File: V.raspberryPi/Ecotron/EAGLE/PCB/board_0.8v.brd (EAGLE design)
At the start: 65.8 x 31.6 mm, 35 parts, among them J1 1X2-3.5MM, J2 1X2-3.5MM, J3 1X2-3.5MM, J4 4P-2.0, J5 4P-2.0, J6 4P-2.0, J7 4P-2.0, T1 T1, T2 T2, T4 MOSFET-N, T6 MOSFET-N, U1 ADS1015, U2 PCA9685, U3 TXB0108, U4 PCA9546APW,112

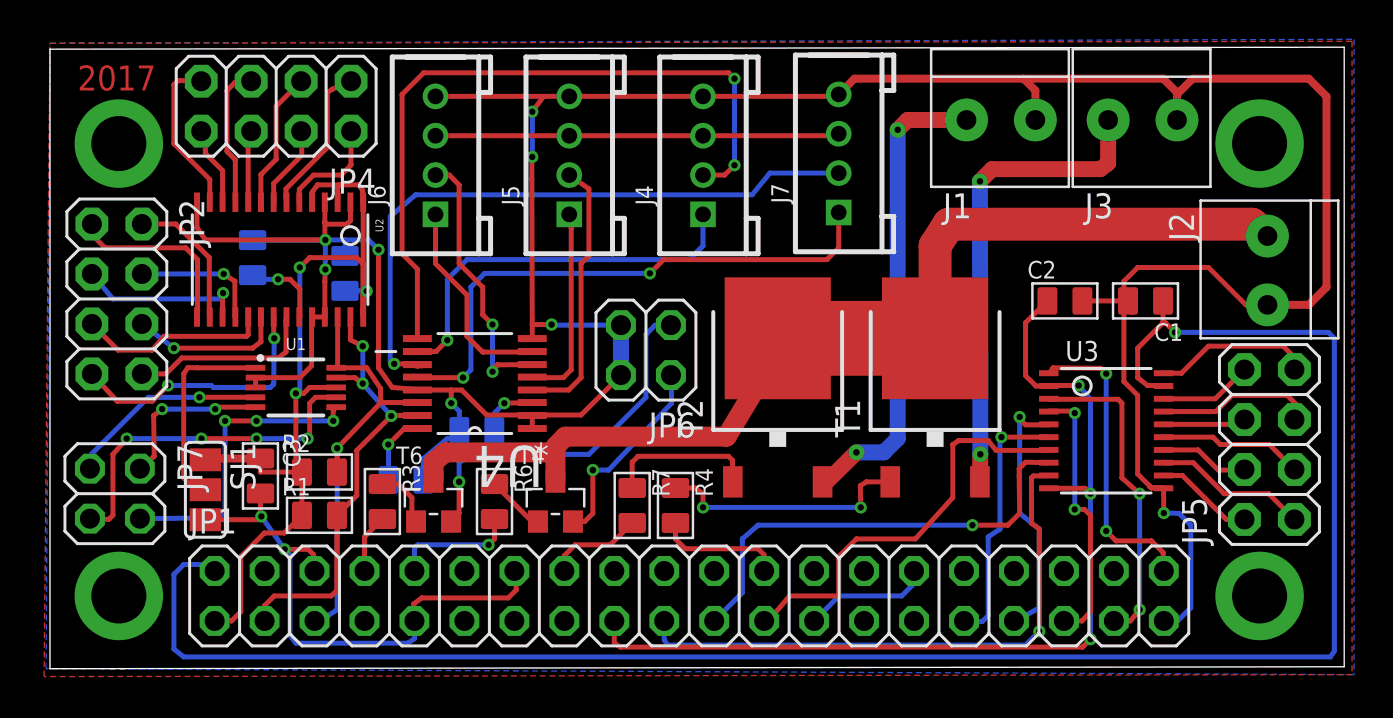
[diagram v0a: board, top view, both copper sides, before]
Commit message: update board
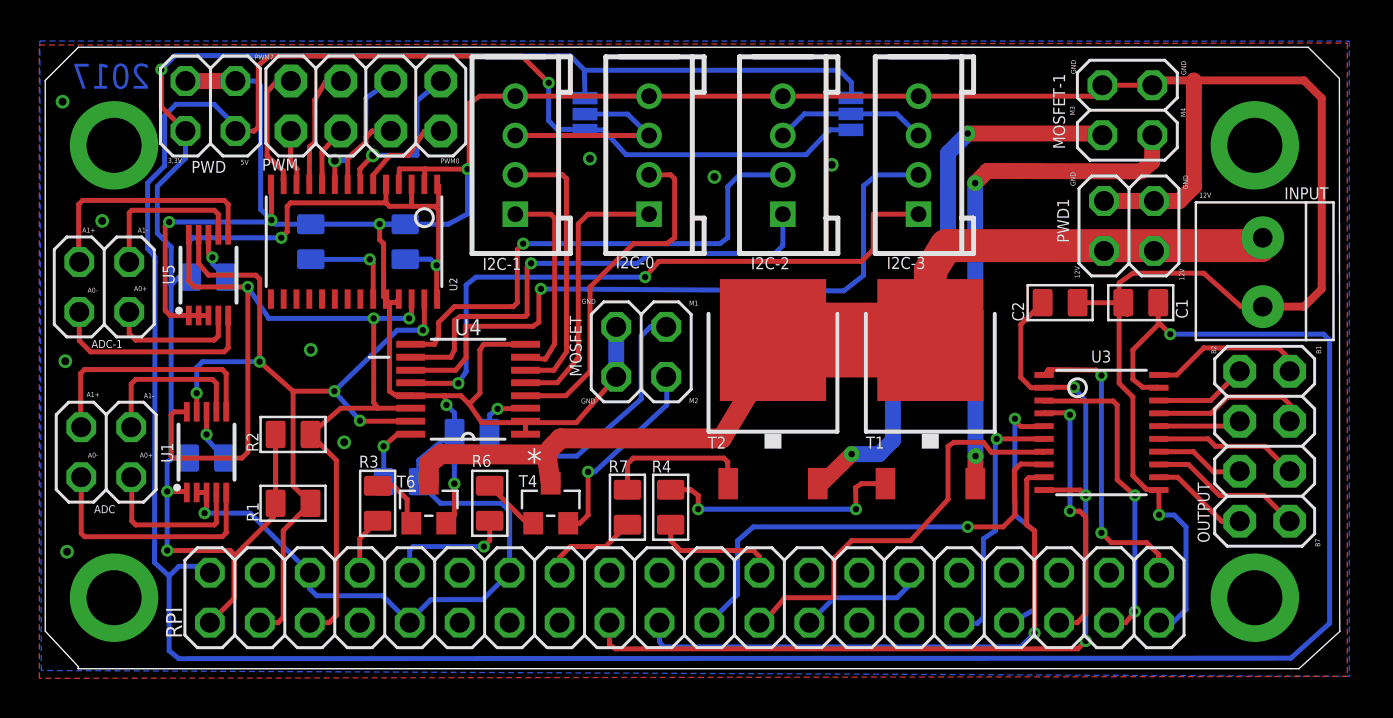
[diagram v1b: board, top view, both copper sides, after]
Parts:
- removed J1, J2, J3: 1X2-3.5MM, adafruit:1X2-3.5MM
- removed J4, J5, J6, J7: 4P-2.0, Seeed-OPL-Connector:HW4-2.0
- removed JP4: PWM, adafruit:2X04
- removed JP5: PINSOUT, adafruit:2X04
- removed JP6: MOSFET, pinhead:2X02
- removed JP7: ADC, pinhead:2X02
- removed SJ1: ADDR, jumper:SJ_2
- removed U$1: 10K, Seeed-OPL-Resistor:R0805
- added ADC, ADC-1, MOSFET-1, PWD, PWD1: (no value), pinhead:2X02
- added C5: 100nf, Seeed-OPL-Capacitor:C0805
- added I2C-0, I2C-1, I2C-2, I2C-3: 4P-2.0, Seeed-OPL-Connector:HW4-2.0
- added INPUT: 1X2-3.5MM, adafruit:1X2-3.5MM
- added MOSFET: MOSFET, pinhead:2X02
- added OUTPUT: PINSOUT, adafruit:2X04
- added PWM: PWM, adafruit:2X04
- added R8: 10K, Seeed-OPL-Resistor:R0805
- added RPI: GPIO, adafruit:2X20
- added U5: ADS1015, SparkFun-IC-Conversion:MSOP10
- C3: value 0.1uf -> 100nf
- JP1: value GPIO -> JUMPER-SMT_3_NO_SILK; device adafruit:2X20 -> SparkFun-Jumpers:SMT-JUMPER_3_NO_SILK
- JP2: value PWM -> JUMPER-SMT_3_NO_SILK; device adafruit:2X04 -> SparkFun-Jumpers:SMT-JUMPER_3_NO_SILK
- moved JP2 38.5 mm to (41.3, 28.6), flipped to the bottom, turned to 90 degrees
- moved JP1 25.1 mm to (27.8, 28.6), flipped to the bottom, turned to 270 degrees
- moved C3 10.5 mm to (8.66, 20.3), flipped to the bottom, turned to 90 degrees
- moved U1 5.61 mm to (8.56, 11.4), turned to 0 degrees
- moved U2 3.87 mm to (16.1, 22.1)
- moved C4 3.46 mm to (18.7, 22.1)
- moved R2 2.33 mm to (13.0, 12.3)
- moved R1 1.47 mm to (13.0, 8.81)
- moved U4 0.45 mm to (21.9, 14.6)
- moved C2 0.26 mm to (52.0, 19.0)
- moved T6 0.26 mm to (19.9, 8.81)
- moved T1 0.26 mm to (45.4, 14.6)
- moved T2 0.26 mm to (37.4, 14.6)
- moved R3 0.26 mm to (17.3, 8.81)
- moved R6 0.26 mm to (23.0, 8.81)
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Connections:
- removed net ADDR_AD: SJ1.2, U1.1
- removed net VCC: J4.3, J5.3, J6.3, J7.3
- new net A0+_1: ADC-1.3, U5.4
- new net A0-_1: ADC-1.1, U5.5
- new net A1+_1: ADC-1.2, U5.6
- new net A1-_1: ADC-1.4, U5.7
- new net N$13: C5.1, U1.8
- new net N$8: C3.1, U5.8
- new net VCC_I2C_1: I2C-0.3, I2C-1.3, JP1.2
- new net VCC_I2C_2: I2C-2.3, I2C-3.3, JP2.2
- net 12V: now also INPUT.1, PWD1.1, PWD1.3; no longer J2.1
- net 3,3V: now also C3.2, C5.2, JP2.3, PWD.1, RPI.1, U1.1; no longer C3.1, SJ1.1, U1.8
- net 3,3V_1: now also RPI.17; no longer JP1.17
- net 5V: now also JP1.3, JP2.1, PWD.3, RPI.2; no longer JP1.2
- net A0+: now also ADC.3; no longer JP7.1
- net A0-: now also ADC.1; no longer JP7.2
- net A1+: now also ADC.2; no longer JP7.4
- net A1-: now also ADC.4; no longer JP7.3
- net B1: now also OUTPUT.7; no longer JP5.7
- net B2: now also OUTPUT.8; no longer JP5.8
- net B3: now also OUTPUT.5; no longer JP5.5
- net B4: now also OUTPUT.6; no longer JP5.6
- net B5: now also OUTPUT.3; no longer JP5.3
- net B6: now also OUTPUT.4; no longer JP5.4
- net B7: now also OUTPUT.1; no longer JP5.1
- net B8: now also OUTPUT.2; no longer JP5.2
- net CLK: now also RPI.7; no longer JP1.7
- net GND: now also I2C-0.4, I2C-1.4, I2C-2.4, I2C-3.4, INPUT.2, MOSFET-1.3, MOSFET-1.4, MOSFET.3, MOSFET.4, PWD.2, PWD.4, PWD1.2, PWD1.4, R8.1, RPI.14, RPI.25, RPI.30, RPI.39, RPI.6, RPI.9, U5.1, U5.2, U5.3; no longer C3.2, J1.2, J2.2, J3.2, J4.4, J5.4, J6.4, J7.4, JP1.14, JP1.25, JP1.30, JP1.39, JP1.6, JP1.9, JP6.3, JP6.4, SJ1.3, U$1.1
- net GND_3: now also RPI.20; no longer JP1.20
- net GND_6: now also RPI.34; no longer JP1.34
- net GPIO10: now also RPI.19; no longer JP1.19
- net GPIO11: now also RPI.23; no longer JP1.23
- net GPIO12: now also RPI.32; no longer JP1.32
- net GPIO13: now also RPI.33; no longer JP1.33
- net GPIO14: now also RPI.8; no longer JP1.8
- net GPIO15: now also RPI.10; no longer JP1.10
- net GPIO16: now also RPI.36; no longer JP1.36
- net GPIO17: now also RPI.11; no longer JP1.11
- net GPIO18: now also RPI.12; no longer JP1.12
- net GPIO19: now also RPI.35; no longer JP1.35
- net GPIO20: now also RPI.38; no longer JP1.38
- net GPIO21: now also RPI.40; no longer JP1.40
- net GPIO22: now also RPI.15; no longer JP1.15
- net GPIO23: now also RPI.16; no longer JP1.16
- net GPIO26: now also RPI.37; no longer JP1.37
- net GPIO27: now also RPI.13; no longer JP1.13
- net GPIO5: now also RPI.29; no longer JP1.29
- net GPIO6: now also RPI.31; no longer JP1.31
- net GPIO7: now also RPI.26; no longer JP1.26
- net GPIO8: now also RPI.24; no longer JP1.24
- net GPIO9: now also RPI.21; no longer JP1.21
- net MOSFET_1: now also MOSFET.1; no longer JP6.1
- net MOSFET_2: now also MOSFET.2; no longer JP6.2
- net MOSFET_3: now also MOSFET-1.2; no longer J1.1
- net MOSFET_4: now also MOSFET-1.1; no longer J3.1
- net N$16: now also R8.2; no longer U$1.2
- net N$23: now also RPI.18; no longer JP1.18
- net N$25: now also RPI.22; no longer JP1.22
- net N$30: now also RPI.27; no longer JP1.27
- net N$38: now also RPI.28; no longer JP1.28
- net N$5: now also RPI.4; no longer JP1.4
- net PWM0: now also PWM.2; no longer JP4.2
- net PWM1: now also PWM.1; no longer JP4.1
- net PWM10: no longer JP2.3
- net PWM11: no longer JP2.4
- net PWM12: no longer JP2.5
- net PWM13: no longer JP2.6
- net PWM14: no longer JP2.7
- net PWM15: no longer JP2.8
- net PWM2: now also PWM.4; no longer JP4.4
- net PWM3: now also PWM.3; no longer JP4.3
- net PWM4: now also PWM.6; no longer JP4.6
- net PWM5: now also PWM.5; no longer JP4.5
- net PWM6: now also PWM.8; no longer JP4.8
- net PWM7: now also PWM.7; no longer JP4.7
- net PWM8: no longer JP2.1
- net PWM9: no longer JP2.2
- net SC0: now also I2C-0.1; no longer J5.1
- net SC1: now also I2C-1.1; no longer J6.1
- net SC2: now also I2C-2.1; no longer J4.1
- net SC3: now also I2C-3.1; no longer J7.1
- net SCL: now also RPI.5, U5.10; no longer JP1.5
- net SD0: now also I2C-0.2; no longer J5.2
- net SD1: now also I2C-1.2; no longer J6.2
- net SD2: now also I2C-2.2; no longer J4.2
- net SD3: now also I2C-3.2; no longer J7.2
- net SDA: now also RPI.3, U5.9; no longer JP1.3
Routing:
- net 5V: track 96.3 -> 162.8 mm, vias 1 -> 2
- net 3,3V: track 48.9 -> 108.0 mm, vias 3 -> 5
- net SCL: track 22.0 -> 52.5 mm, vias 1 -> 3
- net SDA: track 23.5 -> 44.8 mm, vias 3 -> 5
- net VCC: track 20.6 -> 0.00 mm
- net PWM14: track 13.7 -> 0.00 mm, vias 2 -> 0
- net A1+_1: track 0.00 -> 12.3 mm
- net GND: track 208.7 -> 220.9 mm, vias 10 -> 16
- net A0-_1: track 0.00 -> 11.0 mm
- net VCC_I2C_1: track 0.00 -> 10.5 mm
- net ADDR_AD: track 10.5 -> 0.00 mm
- net SD2: track 36.4 -> 26.1 mm, vias 2 -> 1
- net A1-: track 18.0 -> 8.16 mm, vias 4 -> 0
- net PWM12: track 9.76 -> 0.00 mm
- net PWM15: track 9.55 -> 0.00 mm
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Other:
- outline, holes or cut-outs redrawn
- board text added: "12V"
- board text added: "3,3V"
- board text added: "5V"
- board text added: "A0+"
- board text added: "A0-"
- board text added: "A1+"
- board text added: "A1-"
- board text added: "B1"
- board text added: "B2"
- board text added: "B7"
- board text added: "GND"
- board text added: "M1"
- board text added: "M2"
- board text added: "M3"
- board text added: "M4"
- board text added: "PWM0"
- board text added: "PWM7"
